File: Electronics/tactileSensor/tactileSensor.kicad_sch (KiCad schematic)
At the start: 1 part

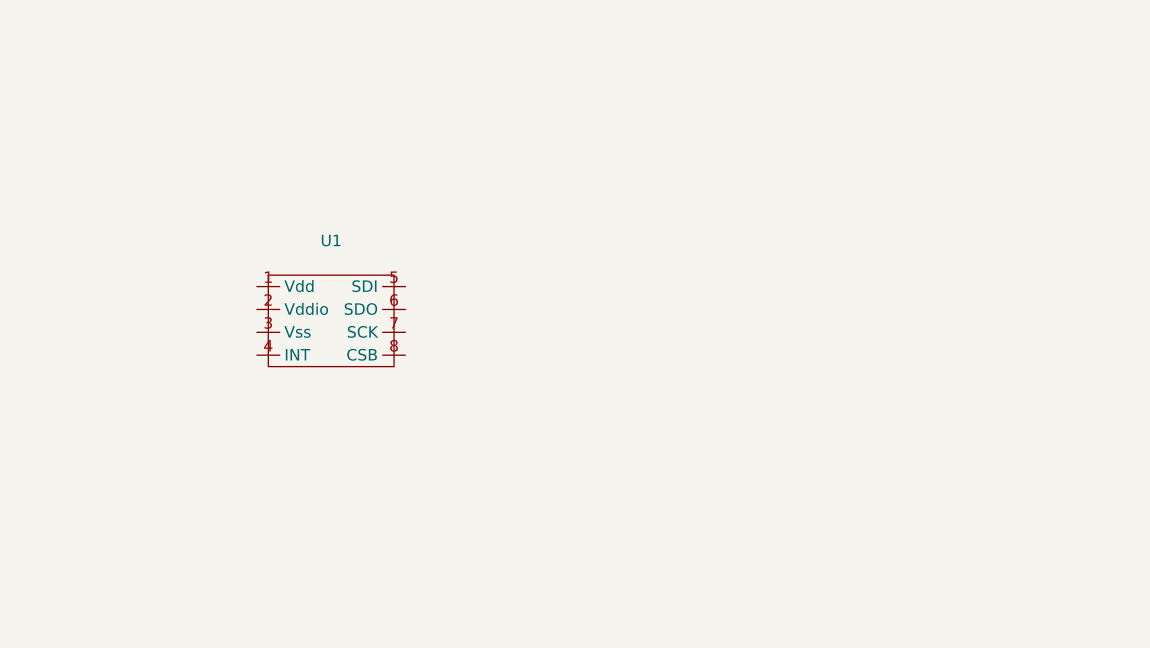
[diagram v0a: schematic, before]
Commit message: ready schematic for board 4Wire SPI
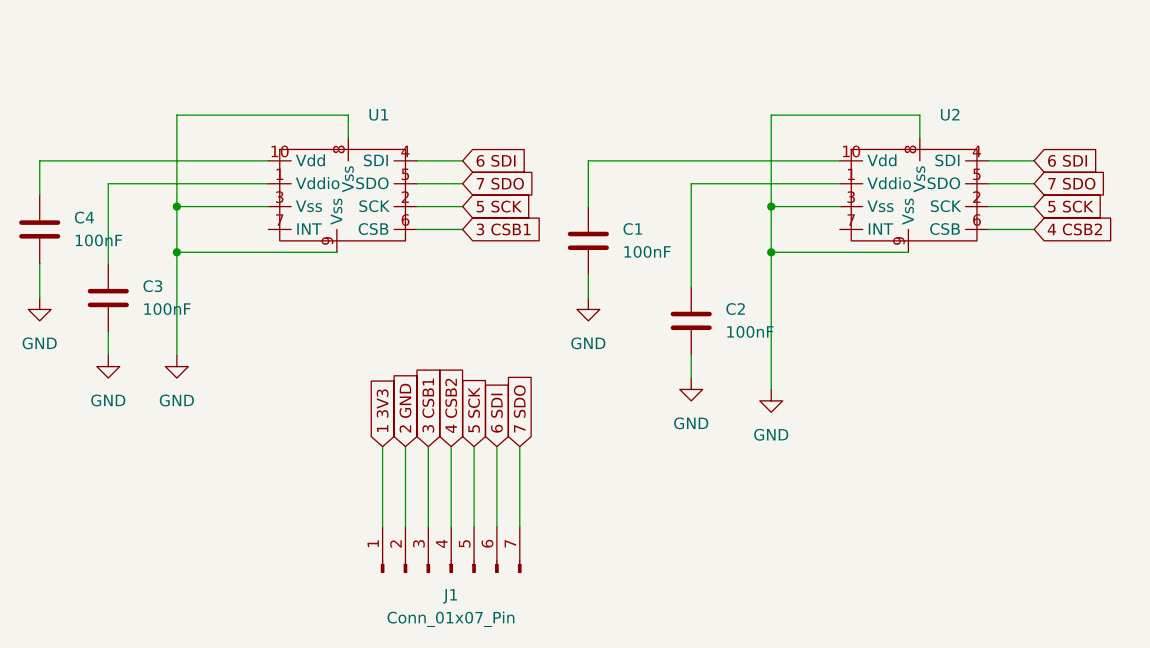
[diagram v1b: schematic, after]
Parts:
- added C1, C2, C3, C4: 100nF, Capacitor_SMD:C_Elec_3x5.4, symbol Device:C
- added J1: Conn_01x07_Pin, symbol Connector:Conn_01x07_Pin
- added U2: ~, Package_LGA:ST_HLGA-10_2x2mm_P0.5mm_LayoutBorder3x2y, symbol Sensor_Pressure:TEST
- U1: footprint (none) -> Package_LGA:ST_HLGA-10_2x2mm_P0.5mm_LayoutBorder3x2y
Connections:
- net at U1.1 (Vddio): now also C3.1
- net 5 SCK: now reaches U1.2 (SCK)
- net 5 SCK: now also J1.5 (Pin_5), U2.2 (SCK)
- net GND: now reaches U1.3 (Vss)
- net GND: now also U1.8 (Vss), U1.9 (Vss), C1.2, C2.2, C3.2, C4.2, U2.3 (Vss), U2.8 (Vss), U2.9 (Vss)
- net 6 SDI: now reaches U1.4 (SDI)
- net 6 SDI: now also J1.6 (Pin_6), U2.4 (SDI)
- net 7 SDO: now reaches U1.5 (SDO)
- net 7 SDO: now also J1.7 (Pin_7), U2.5 (SDO)
- net 3 CSB1: now reaches U1.6 (CSB)
- net 3 CSB1: now also J1.3 (Pin_3)
- new net: C4.1, U1.10 (Vdd)
- new net: C2.1, U2.1 (Vddio)
- new net: C1.1, U2.10 (Vdd)
- new net 1 3V3: J1.1 (Pin_1)
- new net 2 GND: J1.2 (Pin_2)
- new net 4 CSB2: J1.4 (Pin_4), U2.6 (CSB)

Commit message: PCB for mini sensor
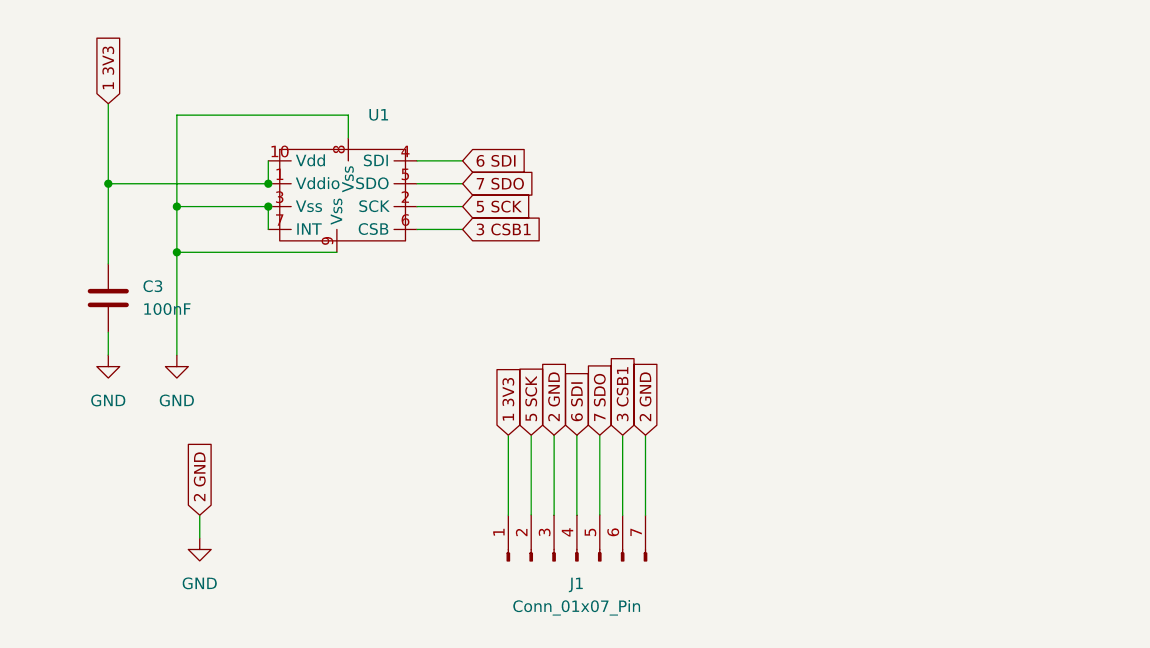
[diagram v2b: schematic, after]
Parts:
- removed C1, C2, C4: 100nF, Capacitor_SMD:C_Elec_3x5.4, symbol Device:C
- removed U2: ~, Package_LGA:ST_HLGA-10_2x2mm_P0.5mm_LayoutBorder3x2y, symbol Sensor_Pressure:TEST
- C3: footprint Capacitor_SMD:C_Elec_3x5.4 -> Capacitor_SMD:C_0805_2012Metric
- J1: footprint (none) -> myOwn:padyBMP581
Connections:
- net 2 GND is gone; now on net 5 SCK: J1.2 (Pin_2)
- net 4 CSB2 is gone; now on net 6 SDI: J1.4 (Pin_4)
- net 1 3V3: now also C3.1, U1.1 (Vddio), U1.10 (Vdd)
- net 3 CSB1: now also J1.6 (Pin_6); no longer J1.3 (Pin_3)
- net 5 SCK: no longer J1.5 (Pin_5)
- net 6 SDI: no longer J1.6 (Pin_6)
- net 7 SDO: now also J1.5 (Pin_5); no longer J1.7 (Pin_7)
- net GND: now also J1.3 (Pin_3), J1.7 (Pin_7), U1.7 (INT)
